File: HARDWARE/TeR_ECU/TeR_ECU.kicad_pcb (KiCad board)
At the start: 4 copper layers, 108.5 x 67.8 mm, 167 parts, among them IC1 MX34040NF2, J1 RJ45_Shielded, J2 RJ45_Shielded, J3 DEBUG, J4 USB_B_Mini, J5 GPS_ANT, K2 G5Q-1, Q1 ZXMN3F30FH, Q2 ZXMN3F30FH, Q3 ZXMN3F30FH, Q4 ZXMN3F30FH, Q5 ZXMN3F30FH, SW1 RST, SW2 BOOT0, U1 TCAN332, U10 NEO-M9N, U11 AT24CS02-STUM, U2 TCAN332, U3 TSR_1-2450, U4 LM1117MP-3.3, U5 LM324, U6 STM32F405VGTx, U7 USBLC6-2SC6, U8 ASM330LHH, U9 LIS3MDL, Y2 ECS-250-20-33-CKM-TR

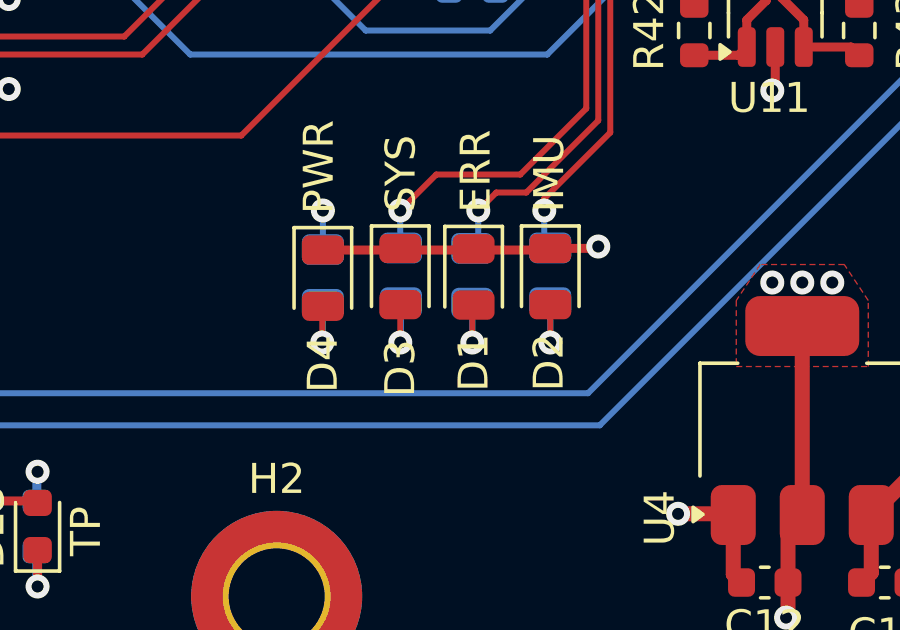
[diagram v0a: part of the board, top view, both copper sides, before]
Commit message: Archivos de producción V2.0.0
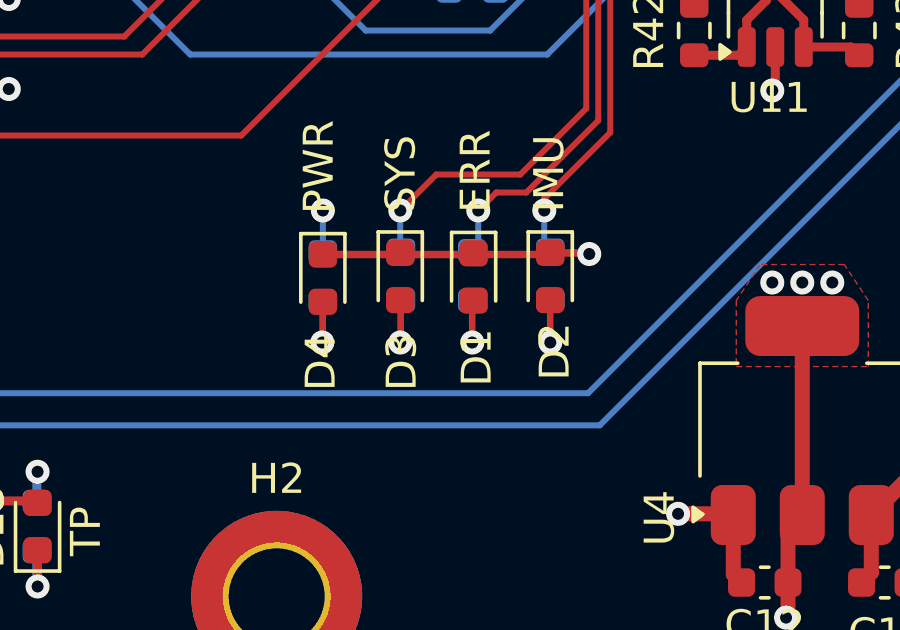
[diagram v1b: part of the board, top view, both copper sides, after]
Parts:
- D1, D2, D3, D4: footprint LED_SMD:LED_0805_2012Metric -> LED_SMD:LED_0603_1608Metric
- R1, R2, R3, R4: footprint Resistor_SMD:R_0805_2012Metric -> Resistor_SMD:R_0603_1608Metric
